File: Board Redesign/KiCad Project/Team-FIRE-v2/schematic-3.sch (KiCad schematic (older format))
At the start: 0 parts

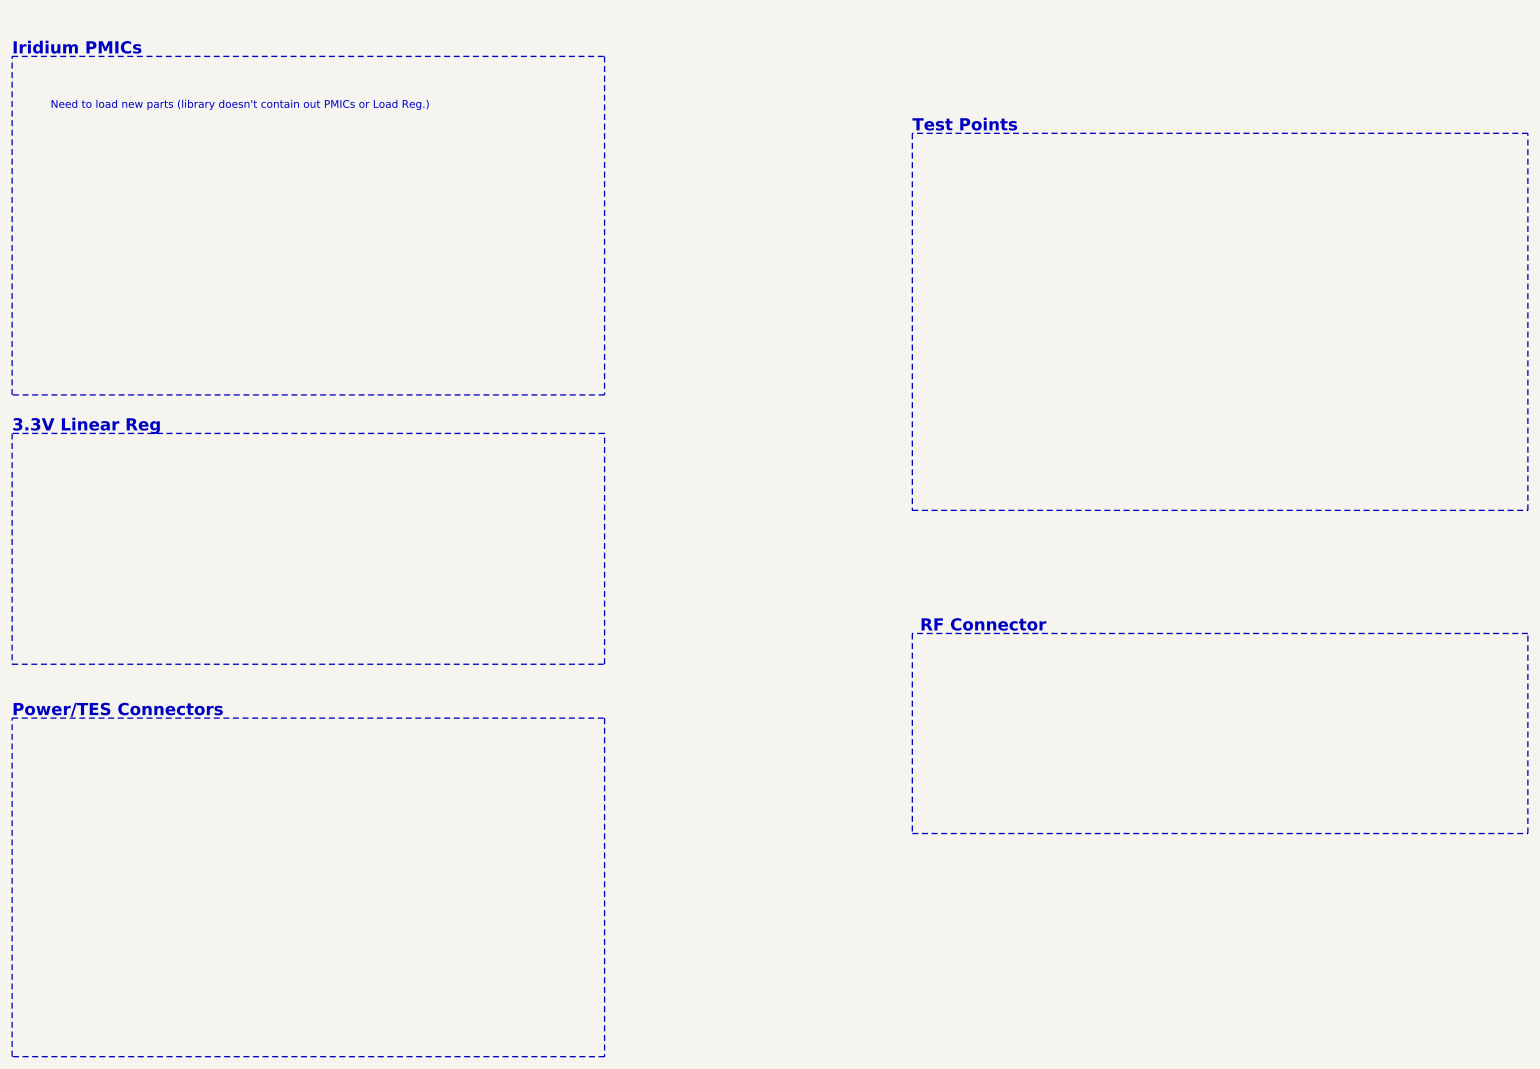
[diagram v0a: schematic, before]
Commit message: Smol changes
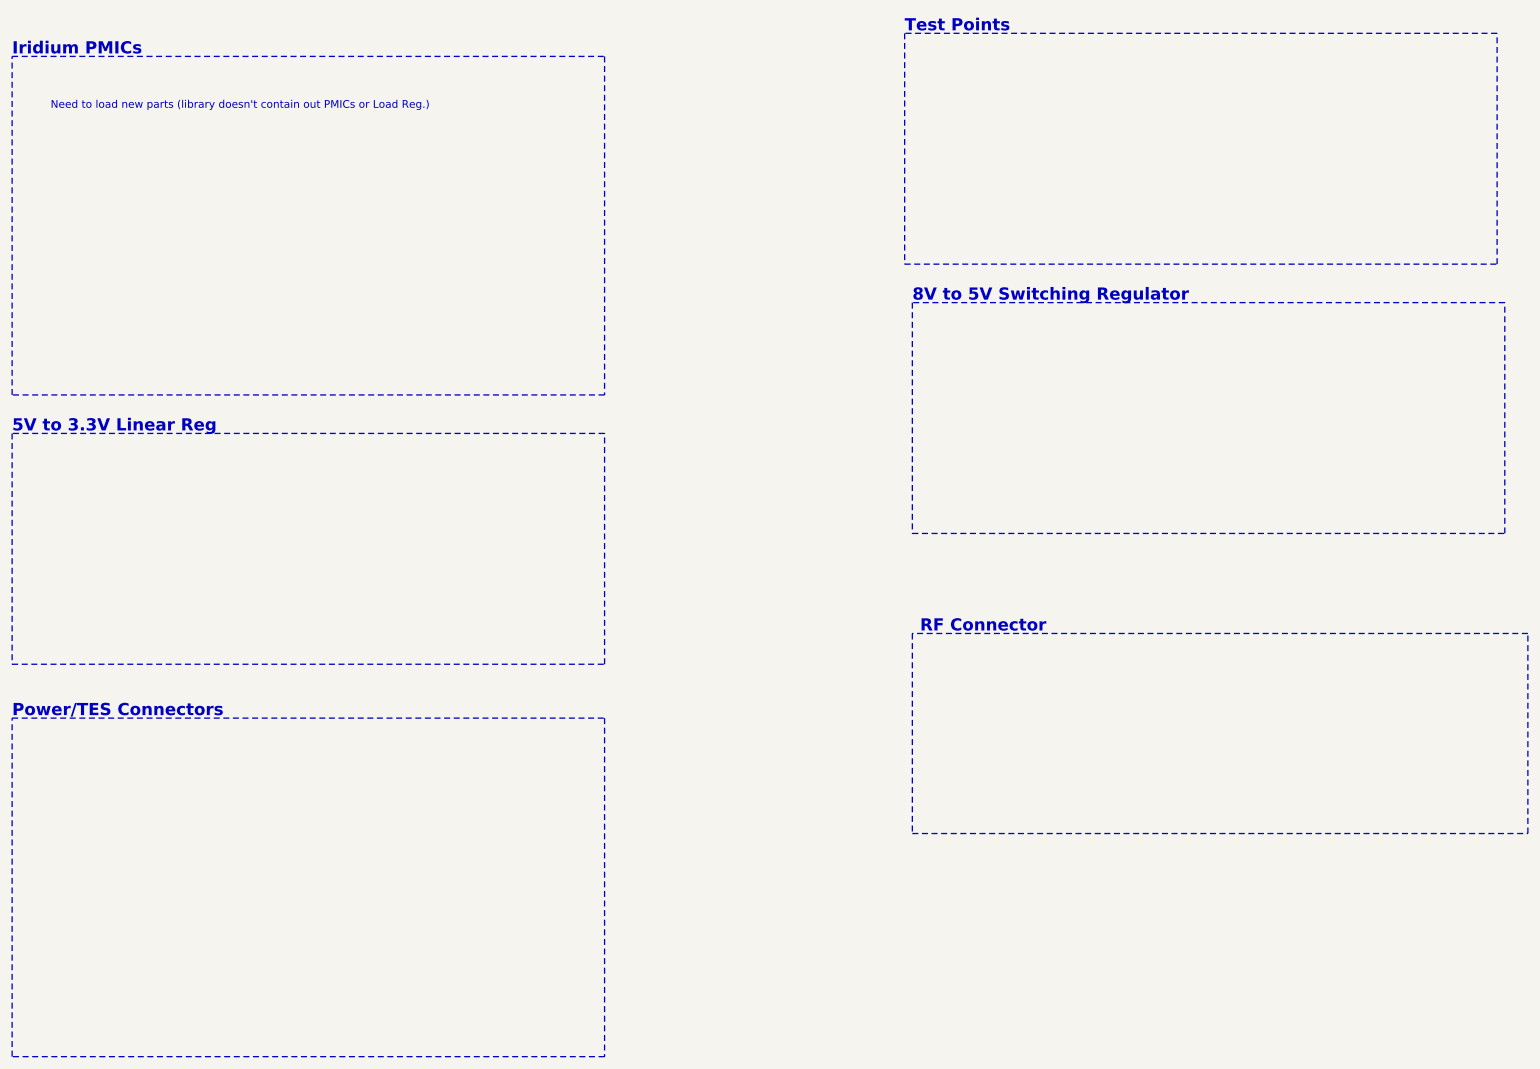
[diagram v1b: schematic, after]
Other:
- note added: "5V to 3.3V Linear Reg"
- note added: "8V to 5V Switching Regulator"
- note removed: "3.3V Linear Reg"
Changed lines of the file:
@@
 EESchema Schematic File Version 4
-LIBS:Team-FIRE-v2-cache
 EELAYER 30 0
 EELAYER END
@@
 Wire Notes Line
 	10900 4750 6900 4750
-Wire Notes Line
-	6900 1500 6900 3950
-Wire Notes Line
-	6900 3950 10900 3950
-Wire Notes Line
-	10900 3950 10900 1500
-Wire Notes Line
-	10900 1500 6900 1500
 Text Notes 6950 4750 0    79   ~ 16
 RF Connector
-Text Notes 6900 1500 0    79   ~ 16
+Text Notes 6850 850  0    79   ~ 16
 Test Points
 Text Notes 1050 1000 0    79   ~ 16
@@
 	4900 3450 1050 3450
 Text Notes 1050 3450 0    79   ~ 16
-3.3V Linear Reg
+5V to 3.3V Linear Reg
 Text Notes 1300 1350 0    50   ~ 0
 Need to load new parts (library doesn't contain out PMICs or Load Reg.)
+Wire Notes Line
+	6900 2600 6900 4100
+Wire Notes Line
+	6900 4100 10750 4100
+Wire Notes Line
+	10750 4100 10750 2600
+Wire Notes Line
+	10750 2600 6900 2600
+Text Notes 6900 2600 0    79   ~ 16
+8V to 5V Switching Regulator
+Wire Notes Line
+	6850 850  6850 2350
+Wire Notes Line
+	6850 2350 10700 2350
+Wire Notes Line
+	10700 2350 10700 850
+Wire Notes Line
+	10700 850  6850 850
 $EndSCHEMATC
